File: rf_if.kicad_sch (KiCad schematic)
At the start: 29 parts, among them U3 Adafruit_Si5351, U4 74LVC74, U5 74HCT244, U6 74HC4066, U7 74HC4066, U8 LM358

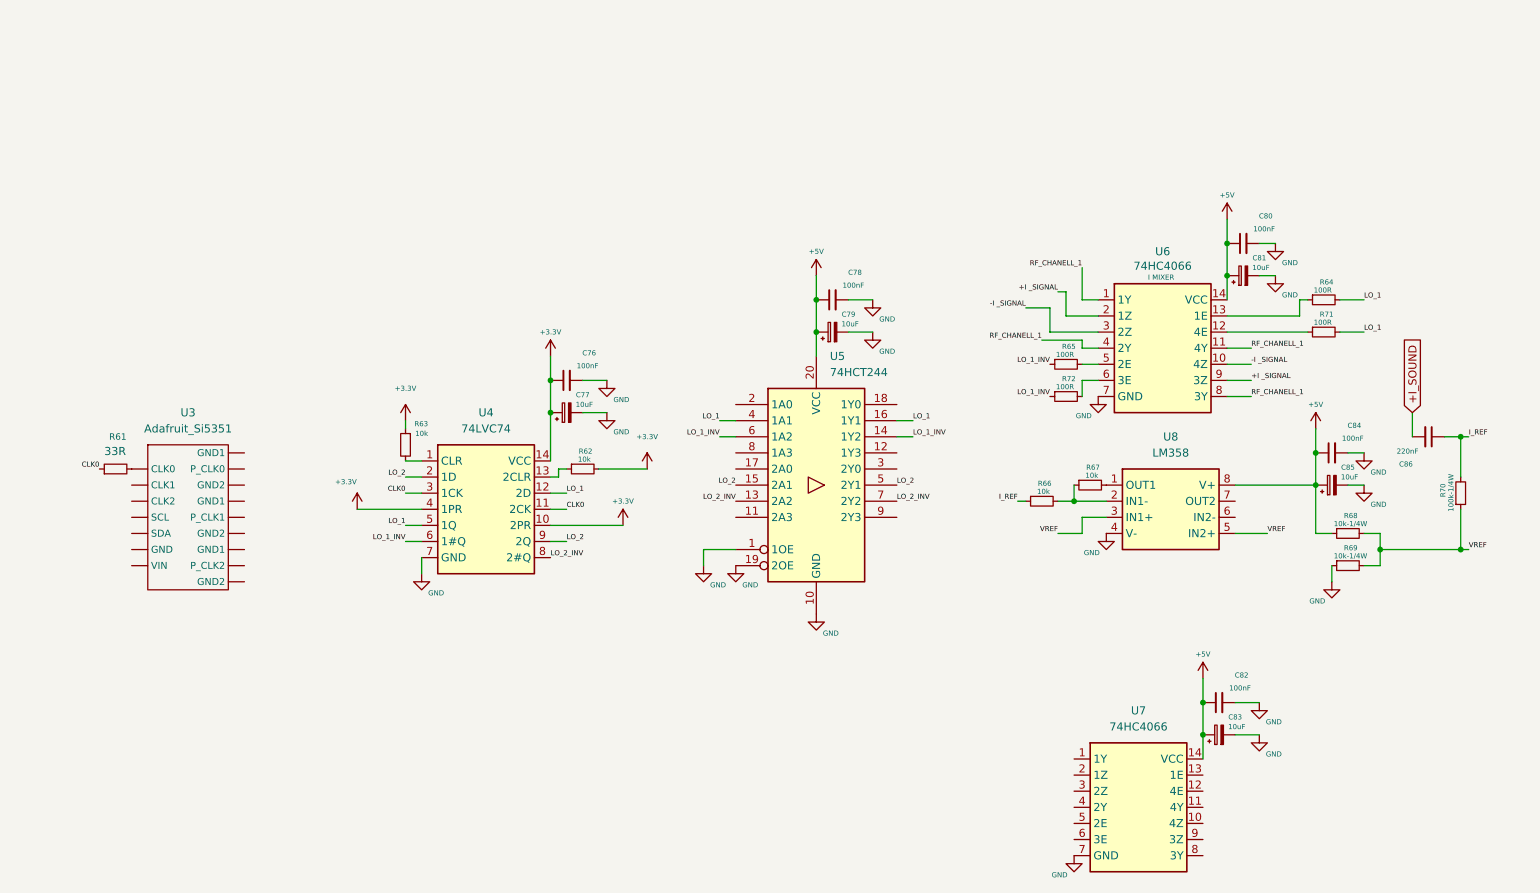
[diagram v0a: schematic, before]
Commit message: Logical Work, Mixers IV
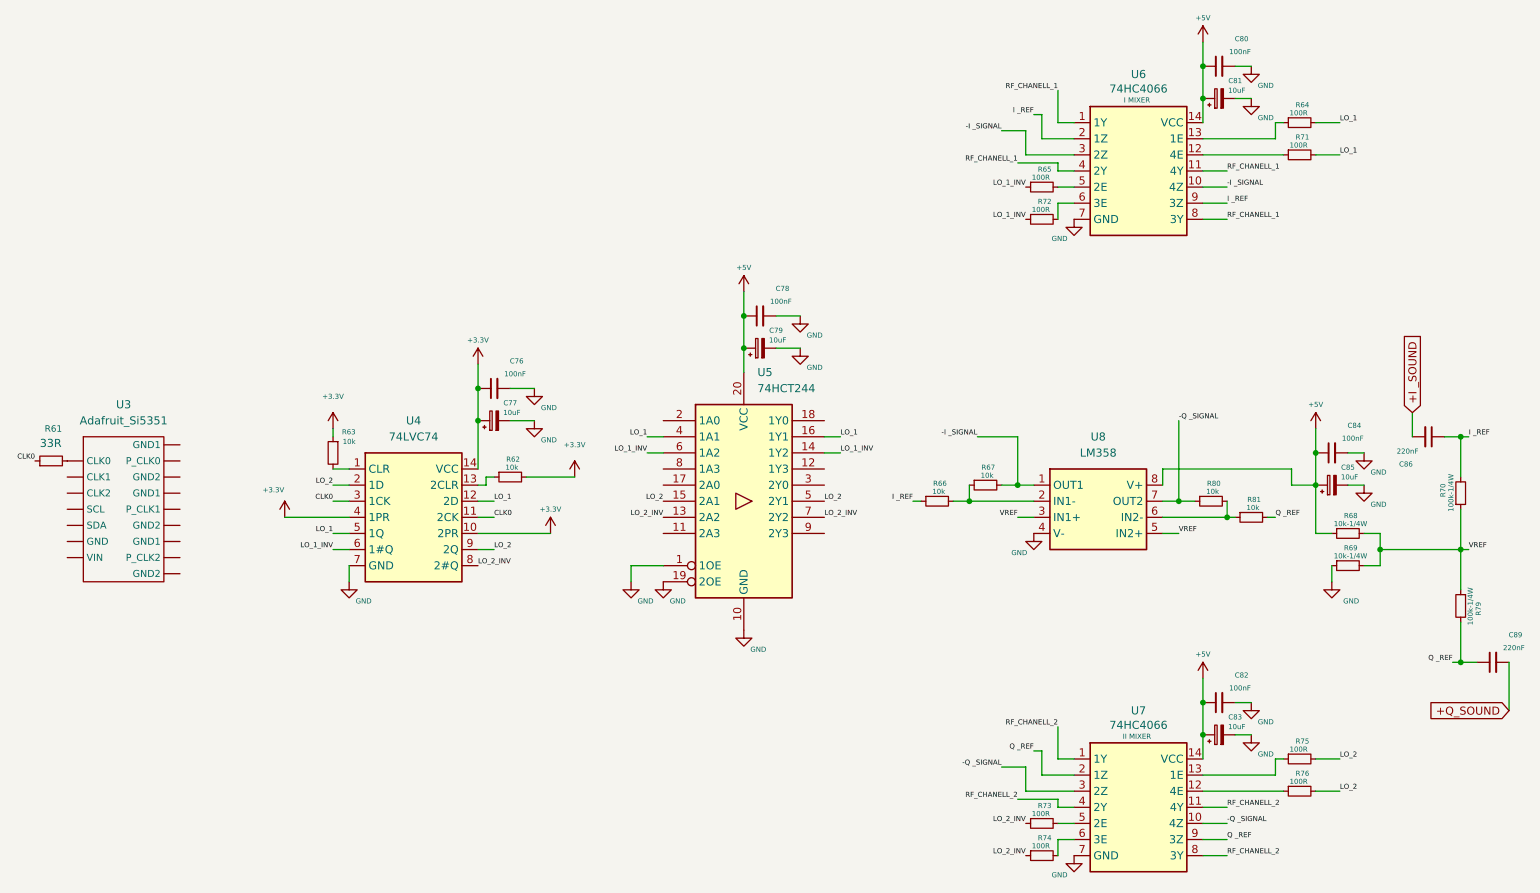
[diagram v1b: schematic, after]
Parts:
- added C89: 220nF, symbol Device:C_Small
- added R73, R74, R75, R76: 100R, symbol Device:R_Small
- added R79: 100k-1/4W, symbol Device:R_Small
- added R80, R81: 10k, symbol Device:R_Small
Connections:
- net I_REF is gone; now on net I _REF: C86.1, R66.1, R70.2
- net -I _SIGNAL: now also R67.2, U8.1 (OUT1)
- net LO_2: now also R75.2, R76.2
- net LO_2_INV: now also R73.1, R74.1
- net VREF: now also R79.1
- net RF_CHANELL_2: now reaches U7.1 (1Y)
- net RF_CHANELL_2: now also U7.11 (4Y), U7.4 (2Y), U7.8 (3Y)
- net -Q _SIGNAL: now reaches U7.10 (4Z)
- net -Q _SIGNAL: now also U7.3 (2Z), U8.7 (OUT2), R80.1
- net at U7.12 (4E): now also R76.1
- net at U7.13 (1E): now also R75.1
- net Q _REF: now reaches U7.2 (1Z)
- net Q _REF: now also U7.9 (3Z), C89.1, R79.2, R81.2
- net at U7.5 (2E): now also R73.2
- net at U7.6 (3E): now also R74.2
- net at U8.6 (IN2-): now also R80.2, R81.1
- net +I _SIGNAL renamed I _REF
- net +I_SOUND renamed +I _SOUND
- new net +Q_SOUND: C89.2
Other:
- note added: "II MIXER"
- moved on the sheet: C76, C77, C78, C79, C80, C81, R61, R62, R63, R64, R65, R66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
